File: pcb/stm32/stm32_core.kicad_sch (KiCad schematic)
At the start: 7 parts

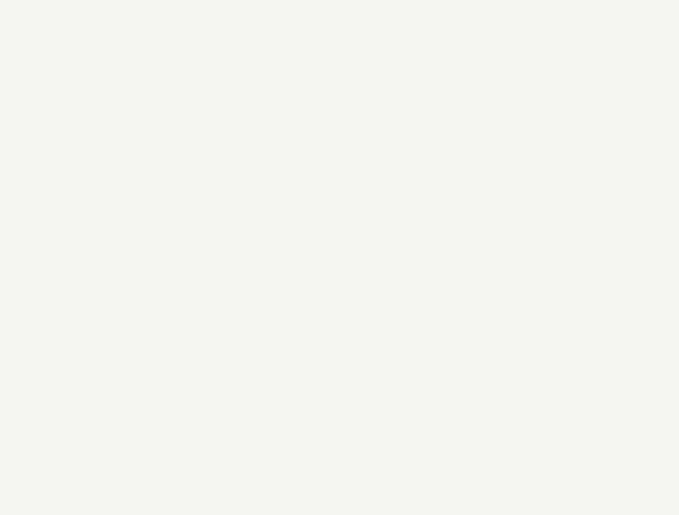
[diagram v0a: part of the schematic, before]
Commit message: Slow progress
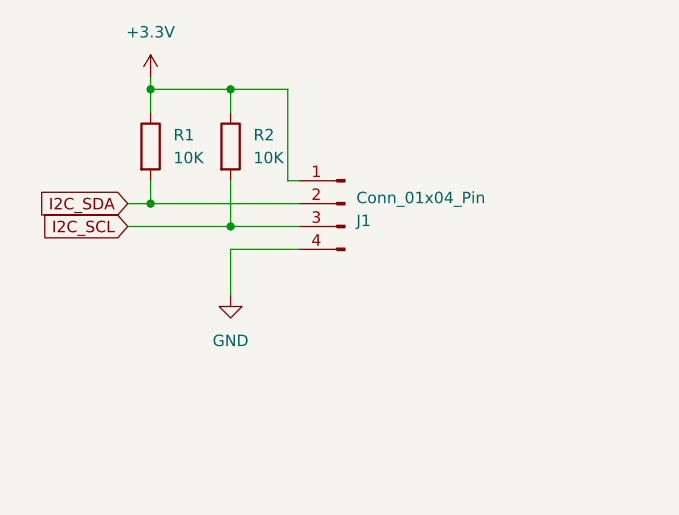
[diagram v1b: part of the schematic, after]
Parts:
- added J1: Conn_01x04_Pin, symbol Connector:Conn_01x04_Pin
- added R1, R2: 10K, symbol Device:R
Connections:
- net +3.3V: now also J1.1 (Pin_1), R1.1, R2.1
- net GND: now also J1.4 (Pin_4)
- net I2C_SCL: now also J1.3 (Pin_3), R2.2
- net I2C_SDA: now also J1.2 (Pin_2), R1.2

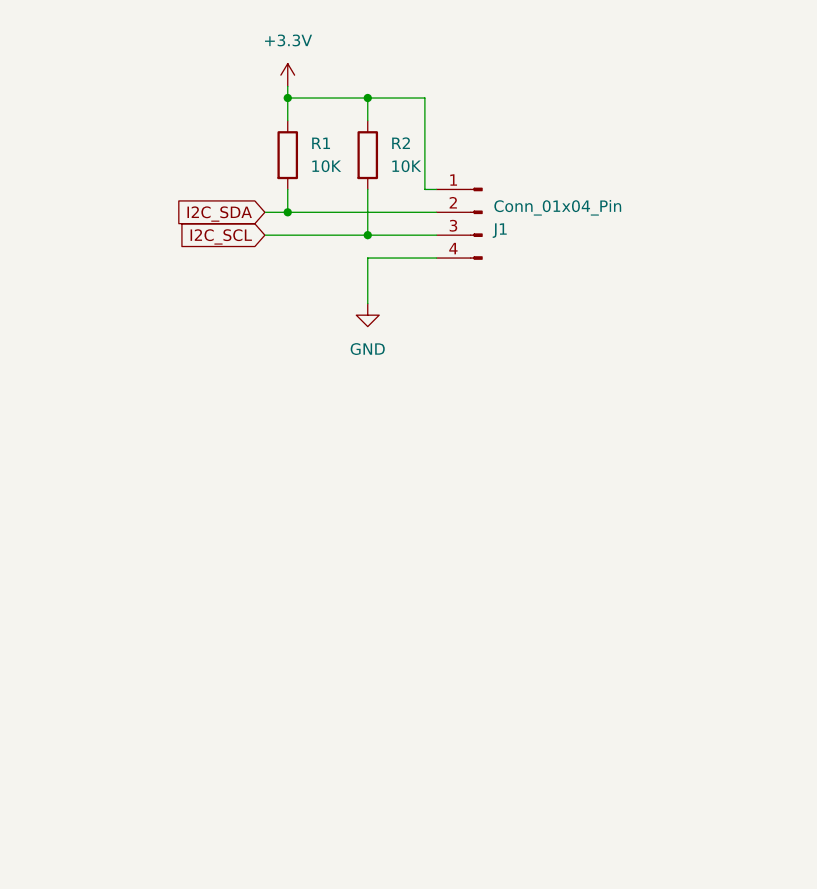
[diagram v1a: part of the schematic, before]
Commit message: Updated PCB
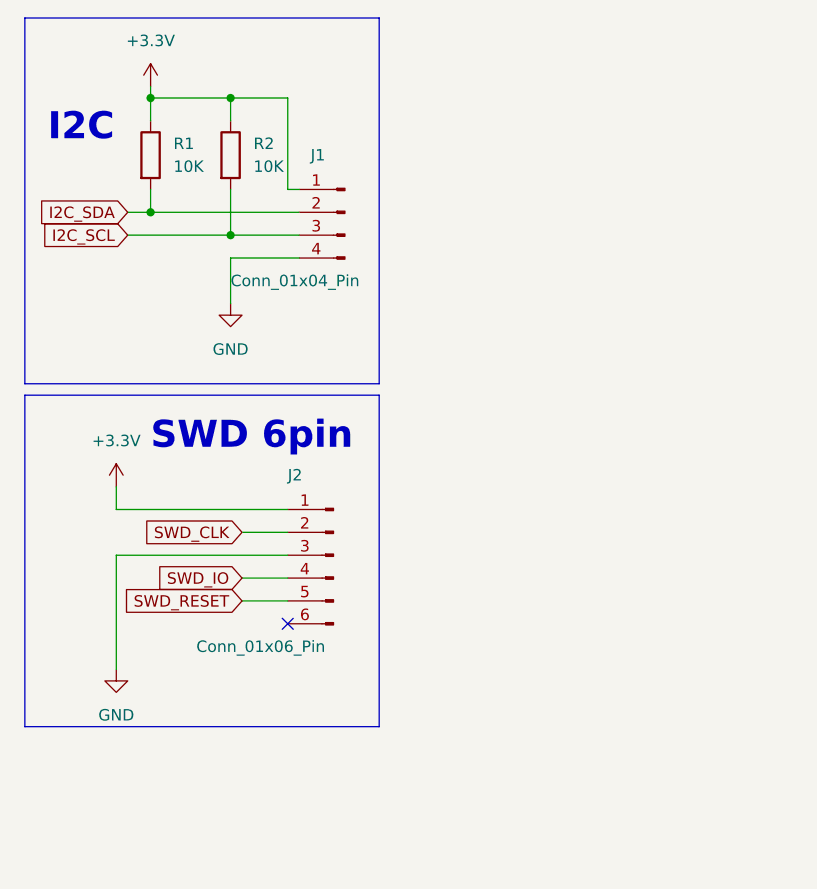
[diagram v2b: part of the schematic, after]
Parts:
- added J2: Conn_01x06_Pin, symbol Connector:Conn_01x06_Pin
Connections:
- net +3.3V: now also J2.1 (Pin_1)
- net BOOT0: now also J2.2 (Pin_2)
- net GND: now also J2.3 (Pin_3)
- net SWD_IO: now also J2.4 (Pin_4)
- net SWD_RESET: now also J2.5 (Pin_5)
- no-connect marks 9 -> 10
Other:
- note added: "I2C"
- note added: "SWD 6pin"
- moved on the sheet: J1, R1, R2
